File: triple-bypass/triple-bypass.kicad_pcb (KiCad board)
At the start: 2 copper layers, 32 x 39.4 mm, 70 parts, among them CON101 MD-90SM, J101 HDR1X2, J102 JMP-PCB-3POS, U101 THS7374IPWR, U102 LMV358M8G-13

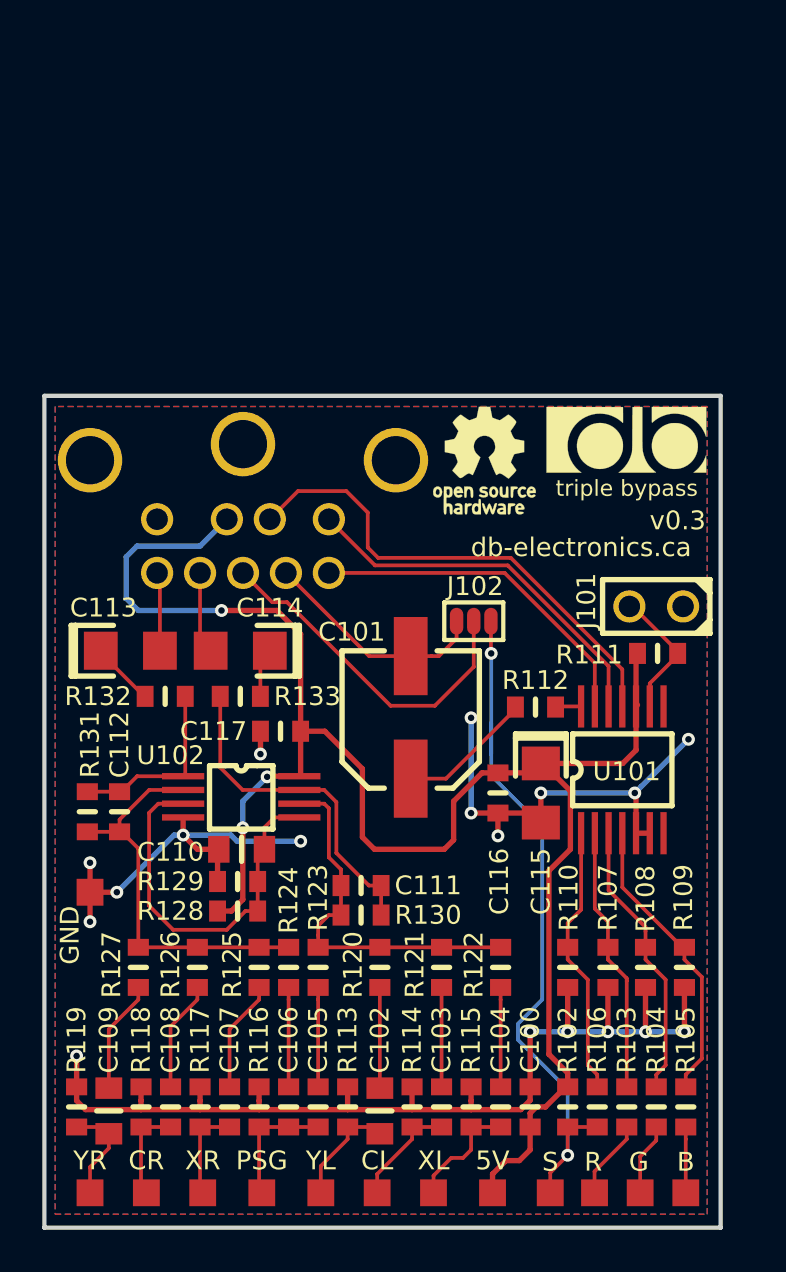
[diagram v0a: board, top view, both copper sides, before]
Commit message: First commit
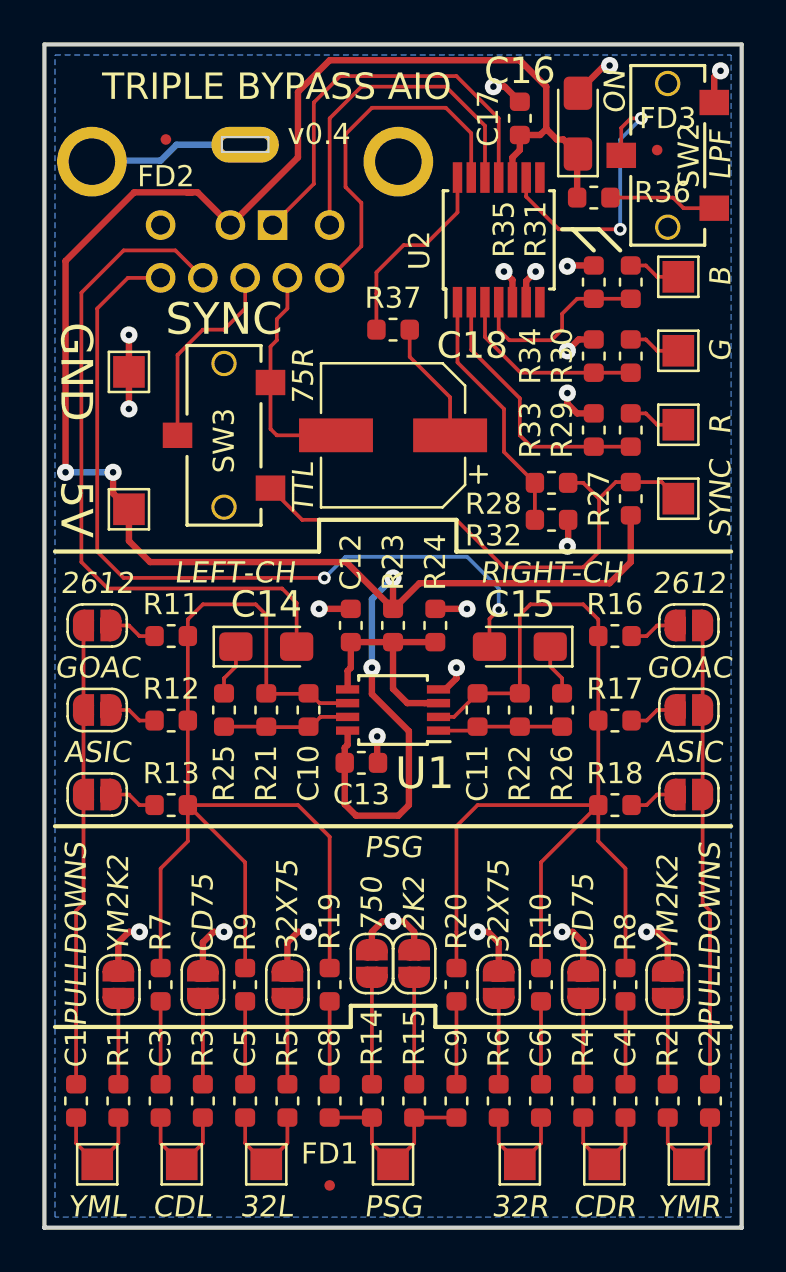
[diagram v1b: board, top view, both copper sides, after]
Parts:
- removed 0V1, 5V1, B1, G1, S1, SL1, SN1, SR2, XL1, XR2, YL1, YR2: TP_50, db-smt:TP50
- removed C100, C116, C117: 0.1uF/50V, db-smt:0603
- removed C101: 220uF/10V, db-smt:SMD-6.6x6.6
- removed C102, C109, C110: 10uF/10V, db-smt:0805
- removed C103, C104, C105, C106, C107, C108: 1uF/16V, db-smt:0603
- removed C111, C112: 270pF/50V, db-smt:0603
- removed C113, C114, C115: 22uF/10V, db-smt:1206_P
- removed CON101: MD-90SM, db-thparts:MD-90SM
- removed G***: LOGO, db-artwork:oshw-logo_5mm
- removed G***: LOGO, db-artwork:db-logo_7.5mm
- removed J101: HDR1X2, db-thparts:HDR1X2
- removed J102: JMP-PCB-3POS, db-smt:JMP-PCB-3POS
- removed R102, R113, R119: 2.20k, db-smt:0603
- removed R103, R104, R105, R106: 5.62k, db-smt:0603
- removed R107, R108, R109, R110: 1.00k, db-smt:0603
- removed R111, R123, R124: 100k, db-smt:0603
- removed R112, R114, R115, R117, R118: 75.0, db-smt:0603
- removed R116: 1.30k, db-smt:0603
- removed R120, R127: 6.19k, db-smt:0603
- removed R121, R122, R125, R126: 130k, db-smt:0603
- removed R128, R129: 10.0k, db-smt:0603
- removed R130, R131: 162k, db-smt:0603
- removed R132, R133: 332, db-smt:0603
- removed U101: THS7374IPWR, db-smt:TSSOP-14
- removed U102: LMV358M8G-13, db-smt:TSSOP-8_3.0mm
- added C1: 10uF/10V, Capacitor_SMD:C_0603_1608Metric, F.Cu at (126.6, 111.6)
- added C10: 180pF/50V, Capacitor_SMD:C_0603_1608Metric, F.Cu at (137.6, 93.1)
- added C11: 180pF/50V, Capacitor_SMD:C_0603_1608Metric, F.Cu at (145.6, 93.1)
- added C12: 10uF/10V, Capacitor_SMD:C_0603_1608Metric, F.Cu at (139.6, 89.1)
- added C13: 0.1uF/50V, Capacitor_SMD:C_0603_1608Metric, F.Cu at (140.1, 95.6)
- added C14: 22uF/10V, Capacitor_Tantalum_SMD:CP_EIA-3216-18_Kemet-A_Pad1.58x1.35mm_HandSolder, F.Cu at (135.6, 90.1)
- added C15: 22uF/10V, Capacitor_Tantalum_SMD:CP_EIA-3216-18_Kemet-A_Pad1.58x1.35mm_HandSolder, F.Cu at (147.6, 90.1)
- added C16: 22uF/10V, Capacitor_Tantalum_SMD:CP_EIA-3216-18_Kemet-A_Pad1.58x1.35mm_HandSolder, F.Cu at (150.3, 65.4)
- added C17: 0.1uF/50V, Capacitor_SMD:C_0603_1608Metric, F.Cu at (147.6, 65.1)
- added C18: 220uF/10V, Capacitor_SMD:CP_Elec_6.3x5.4_Nichicon, F.Cu at (141.6, 80.1)
- added C2: 10uF/10V, Capacitor_SMD:C_0603_1608Metric, F.Cu at (156.6, 111.6)
- added C3: 1uF/16V, Capacitor_SMD:C_0603_1608Metric, F.Cu at (130.6, 111.6)
- added C4: 1uF/16V, Capacitor_SMD:C_0603_1608Metric, F.Cu at (152.6, 111.6)
- added C5: 1uF/16V, Capacitor_SMD:C_0603_1608Metric, F.Cu at (134.6, 111.6)
- added C6: 1uF/16V, Capacitor_SMD:C_0603_1608Metric, F.Cu at (148.6, 111.6)
- added C8: 1uF/16V, Capacitor_SMD:C_0603_1608Metric, F.Cu at (138.6, 111.6)
- added C9: 1uF/16V, Capacitor_SMD:C_0603_1608Metric, F.Cu at (144.6, 111.6)
- added FD1: Fiducial, Fiducial:Fiducial_0.5mm_Dia_1mm_Outer, F.Cu at (138.6, 115.6)
- added FD2: Fiducial, Fiducial:Fiducial_0.5mm_Dia_1mm_Outer, F.Cu at (130.8, 66.1)
- added FD3: Fiducial, Fiducial:Fiducial_0.5mm_Dia_1mm_Outer, F.Cu at (154.1, 66.6)
- added J1: MD-90SM, CUI_MD-90SM, B.Cu at (134.6, 66.4)
- added JP1: SolderJumper_3_Open, Jumper:SolderJumper-2_P1.3mm_Open_RoundedPad1.0x1.5mm, F.Cu at (128.6, 106.1)
- added JP10: SolderJumper_3_Open, Jumper:SolderJumper-2_P1.3mm_Open_RoundedPad1.0x1.5mm, F.Cu at (127.6, 97.1)
- added JP11: SolderJumper_3_Open, Jumper:SolderJumper-2_P1.3mm_Open_RoundedPad1.0x1.5mm, F.Cu at (155.6, 89.1)
- added JP12: SolderJumper_3_Open, Jumper:SolderJumper-2_P1.3mm_Open_RoundedPad1.0x1.5mm, F.Cu at (155.6, 93.1)
- added JP13: SolderJumper_3_Open, Jumper:SolderJumper-2_P1.3mm_Open_RoundedPad1.0x1.5mm, F.Cu at (155.6, 97.1)
- added JP14: SolderJumper_3_Open, Jumper:SolderJumper-2_P1.3mm_Open_RoundedPad1.0x1.5mm, F.Cu at (142.6, 105.1)
- added JP2: SolderJumper_3_Open, Jumper:SolderJumper-2_P1.3mm_Open_RoundedPad1.0x1.5mm, F.Cu at (154.6, 106.1)
- added JP3: SolderJumper_3_Open, Jumper:SolderJumper-2_P1.3mm_Open_RoundedPad1.0x1.5mm, F.Cu at (132.6, 106.1)
- added JP4: SolderJumper_3_Open, Jumper:SolderJumper-2_P1.3mm_Open_RoundedPad1.0x1.5mm, F.Cu at (150.6, 106.1)
- added JP5: SolderJumper_3_Open, Jumper:SolderJumper-2_P1.3mm_Open_RoundedPad1.0x1.5mm, F.Cu at (136.6, 106.1)
- added JP6: SolderJumper_3_Open, Jumper:SolderJumper-2_P1.3mm_Open_RoundedPad1.0x1.5mm, F.Cu at (146.6, 106.1)
- added JP7: SolderJumper_3_Open, Jumper:SolderJumper-2_P1.3mm_Open_RoundedPad1.0x1.5mm, F.Cu at (140.6, 105.1)
- added JP8: SolderJumper_3_Open, Jumper:SolderJumper-2_P1.3mm_Open_RoundedPad1.0x1.5mm, F.Cu at (127.6, 89.1)
- added JP9: SolderJumper_3_Open, Jumper:SolderJumper-2_P1.3mm_Open_RoundedPad1.0x1.5mm, F.Cu at (127.6, 93.1)
- added LOGO1: Logo_Open_Hardware_Small, Symbol:OSHW-Logo2_7.3x6mm_SilkScreen, B.Cu at (141.6, 106.6)
- added P1: TP_50, TestPoint:TestPoint_Pad_1.5x1.5mm, F.Cu at (129.1, 83.6)
- added P10: TP_50, TestPoint:TestPoint_Pad_1.5x1.5mm, F.Cu at (147.6, 114.6)
- added P11: TP_50, TestPoint:TestPoint_Pad_1.5x1.5mm, F.Cu at (131.6, 114.6)
- added P12: TP_50, TestPoint:TestPoint_Pad_1.5x1.5mm, F.Cu at (151.6, 114.6)
- added P13: TP_50, TestPoint:TestPoint_Pad_1.5x1.5mm, F.Cu at (141.6, 114.6)
- added P2: TP_50, TestPoint:TestPoint_Pad_1.5x1.5mm, F.Cu at (129.1, 77.1)
- added P3: TP_50, TestPoint:TestPoint_Pad_1.5x1.5mm, F.Cu at (155.1, 79.6)
- added P4: TP_50, TestPoint:TestPoint_Pad_1.5x1.5mm, F.Cu at (155.1, 76.1)
- added P5: TP_50, TestPoint:TestPoint_Pad_1.5x1.5mm, F.Cu at (155.1, 72.6)
- added P6: TP_50, TestPoint:TestPoint_Pad_1.5x1.5mm, F.Cu at (155.1, 83.1)
- added P7: TP_50, TestPoint:TestPoint_Pad_1.5x1.5mm, F.Cu at (127.6, 114.6)
- added P8: TP_50, TestPoint:TestPoint_Pad_1.5x1.5mm, F.Cu at (155.6, 114.6)
- added P9: TP_50, TestPoint:TestPoint_Pad_1.5x1.5mm, F.Cu at (135.6, 114.6)
- added R10: 130K, Resistor_SMD:R_0603_1608Metric, F.Cu at (148.6, 106.1)
- added R11: 6K19, Resistor_SMD:R_0603_1608Metric, F.Cu at (131.1, 89.6)
- added R12: 43K, Resistor_SMD:R_0603_1608Metric, F.Cu at (131.1, 93.6)
- added R13: 56K, Resistor_SMD:R_0603_1608Metric, F.Cu at (131.1, 97.6)
- added R14: 750R, Resistor_SMD:R_0603_1608Metric, F.Cu at (140.6, 111.6)
- added R15: 2K2, Resistor_SMD:R_0603_1608Metric, F.Cu at (142.6, 111.6)
- added R16: 6K19, Resistor_SMD:R_0603_1608Metric, F.Cu at (152.1, 89.6)
- added R17: 43K, Resistor_SMD:R_0603_1608Metric, F.Cu at (152.1, 93.6)
- added R18: 56K, Resistor_SMD:R_0603_1608Metric, F.Cu at (152.1, 97.6)
- added R19: 120K, Resistor_SMD:R_0603_1608Metric, F.Cu at (138.6, 106.1)
- added R2: 2K2, Resistor_SMD:R_0603_1608Metric, F.Cu at (154.6, 111.6)
- added R20: 120K, Resistor_SMD:R_0603_1608Metric, F.Cu at (144.6, 106.1)
- added R21: 240K, Resistor_SMD:R_0603_1608Metric, F.Cu at (135.6, 93.1)
- added R22: 240K, Resistor_SMD:R_0603_1608Metric, F.Cu at (147.6, 93.1)
- added R23: 10K, Resistor_SMD:R_0603_1608Metric, F.Cu at (141.6, 89.1)
- added R24: 10K, Resistor_SMD:R_0603_1608Metric, F.Cu at (143.6, 89.1)
- added R25: 332R, Resistor_SMD:R_0603_1608Metric, F.Cu at (133.6, 93.1)
- added R26: 332R, Resistor_SMD:R_0603_1608Metric, F.Cu at (149.6, 93.1)
- added R27: 2K2, Resistor_SMD:R_0603_1608Metric, F.Cu at (152.8, 83.1)
- added R28: 5K62, Resistor_SMD:R_0603_1608Metric, F.Cu at (149.1, 82.4)
- added R29: 5K62, Resistor_SMD:R_0603_1608Metric, F.Cu at (152.8, 79.9)
- added R3: 75R, Resistor_SMD:R_0603_1608Metric, F.Cu at (132.6, 111.6)
- added R30: 5K62, Resistor_SMD:R_0603_1608Metric, F.Cu at (152.8, 76.4)
- added R31: 5K62, Resistor_SMD:R_0603_1608Metric, F.Cu at (152.8, 72.9)
- added R32: 1K, Resistor_SMD:R_0603_1608Metric, F.Cu at (149.1, 84.1)
- added R33: 1K, Resistor_SMD:R_0603_1608Metric, F.Cu at (151.1, 79.9)
- added R34: 1K, Resistor_SMD:R_0603_1608Metric, F.Cu at (151.1, 76.4)
- added R35: 1K, Resistor_SMD:R_0603_1608Metric, F.Cu at (151.1, 72.9)
- added R36: 100K, Resistor_SMD:R_0603_1608Metric, F.Cu at (151.1, 68.9)
- added R37: 75R, Resistor_SMD:R_0603_1608Metric, F.Cu at (141.6, 75.1)
- added R4: 75R, Resistor_SMD:R_0603_1608Metric, F.Cu at (150.6, 111.6)
- added R5: 75R, Resistor_SMD:R_0603_1608Metric, F.Cu at (136.6, 111.6)
- added R6: 75R, Resistor_SMD:R_0603_1608Metric, F.Cu at (146.6, 111.6)
- added R7: 130K, Resistor_SMD:R_0603_1608Metric, F.Cu at (130.6, 106.1)
- added R8: 130K, Resistor_SMD:R_0603_1608Metric, F.Cu at (152.6, 106.1)
- added R9: 130K, Resistor_SMD:R_0603_1608Metric, F.Cu at (134.6, 106.1)
- added SW2: SW_SPDT, 100:CL-SB-12B-01, F.Cu at (154.6, 66.9)
- added SW3: SW_SPDT, 100:CL-SB-12B-01, F.Cu at (133.6, 80.1)
- added U1: LMV358M8G-13, Package_SO:TSSOP-8_3x3mm_P0.65mm, F.Cu at (141.6, 93.1)
- added U2: THS7374IPWR, Package_SO:TSSOP-14_4.4x5mm_P0.65mm, F.Cu at (146.6, 70.9)
- R1: value TP_50 -> 2K2; footprint db-smt:TP50 -> Resistor_SMD:R_0603_1608Metric
- moved R1 23.0 mm to (128.6, 111.6), turned to 90 degrees
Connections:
- R1 pad 1: /R-In -> /Mega Amp/YM-LEFT-IN
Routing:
- net /Mega Amp/R-CH: track 0.00 -> 51.9 mm
- net /Mega Amp/L-CH: track 0.00 -> 51.3 mm
- net GND: track 90.0 -> 50.8 mm, vias 18 -> 22
- net /SR: track 3.74 -> 38.6 mm, vias 0 -> 2
- net /SYNC-TTL: track 34.1 -> 0.00 mm, vias 2 -> 0
- net /SL: track 3.89 -> 32.9 mm
- net /Video Amp/SYNC-IN: track 0.00 -> 26.1 mm
- net Net-(C2-Pad1): track 0.00 -> 21.9 mm
- net Net-(C1-Pad1): track 0.00 -> 21.9 mm
- net +5V: track 84.1 -> 104.5 mm, vias 3 -> 4
- net Net-(C112-Pad1): track 18.8 -> 0.00 mm
- net Net-(C110-Pad2): track 18.1 -> 0.00 mm
- net Net-(C111-Pad1): track 18.1 -> 0.00 mm
- net Net-(C111-Pad2): track 16.1 -> 0.00 mm
- net Net-(SW2-Pad2): track 0.00 -> 14.1 mm, vias 0 -> 2
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- removed copper zone on F.Cu, net GND
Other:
- board size 32 x 39.4 mm -> 33 x 56 mm
- net class Power: clearance 0.1778 -> 0.254; trace_width 0.254 -> 0.3048; via_dia 0.6096 -> 0.8128
- board text added: "2612"
- board text added: "2K2"
- board text added: "32L"
- board text added: "32R"
- board text added: "32X75"
- board text added: "750"
- board text added: "75R"
- board text added: "ASIC"
- board text added: "CD75"
- board text added: "CDL"
- board text added: "CDR"
- board text added: "GOAC"
- board text added: "LEFT-CH"
- board text added: "LPF"
- board text added: "ON"
- board text added: "PULLDOWNS"
- board text added: "RIGHT-CH"
- board text added: "SYNC"
- board text added: "TRIPLE BYPASS AIO"
- board text added: "TTL"
- board text added: "YM2K2"
- board text added: "YML"
- board text added: "YMR"
- board text added: "v0.4"
- board text removed: "CL"
- board text removed: "CR"
- board text removed: "S"
- board text removed: "XL"
- board text removed: "XR"
- board text removed: "YL"
- board text removed: "YR"
- board text removed: "db-electronics.ca"
- board text removed: "triple bypass"
- board text removed: "v0.3"
